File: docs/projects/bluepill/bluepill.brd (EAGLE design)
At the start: 89.8 x 49.5 mm, 10 parts

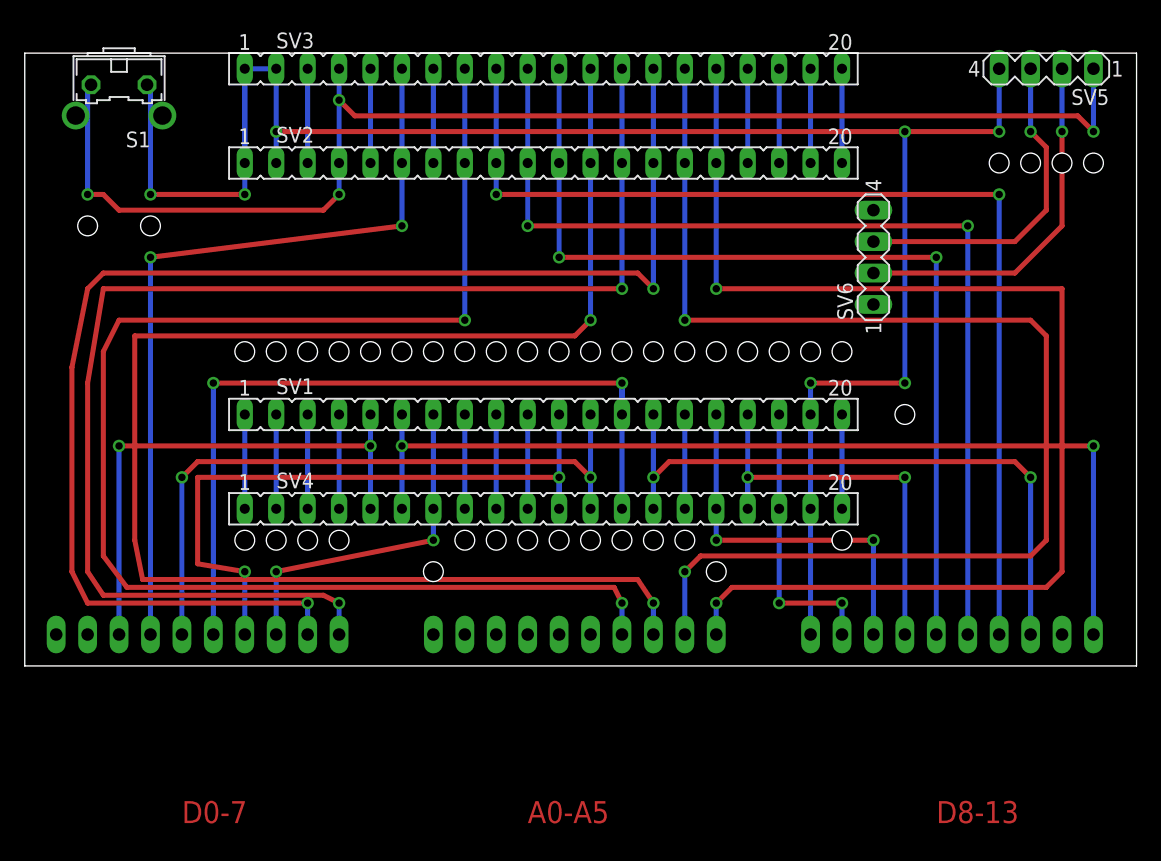
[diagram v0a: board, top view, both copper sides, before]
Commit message: bluepill
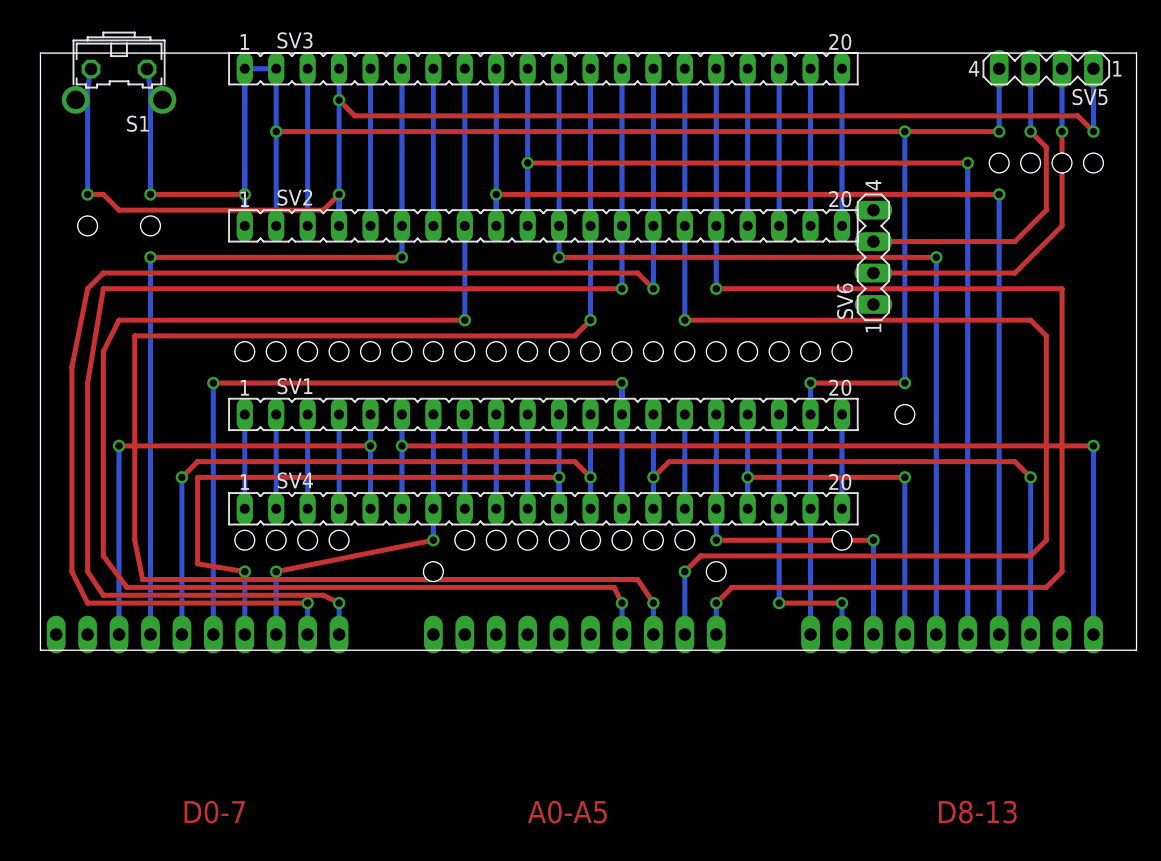
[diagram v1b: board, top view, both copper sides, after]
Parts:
- moved SV2 5.08 mm to (41.9, 35.6)
- moved S1 1.27 mm to (7.62, 47.0)
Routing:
- net GND: track 156.3 -> 167.6 mm
- net D12: track 81.3 -> 91.4 mm
- net RESET: track 107.6 -> 113.9 mm
- net D11: track 86.4 -> 91.4 mm
- net N$8: track 7.62 -> 12.7 mm
- net N$7: track 7.62 -> 12.7 mm
- net N$6: track 7.62 -> 12.7 mm
- net N$5: track 7.62 -> 12.7 mm
- net N$4: track 7.62 -> 12.7 mm
- net N$3: track 7.62 -> 12.7 mm
- net N$1: track 7.62 -> 12.7 mm
- net D6: track 63.7 -> 66.0 mm
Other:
- board size 89.8 x 49.5 mm -> 88.6 x 48.2 mm
